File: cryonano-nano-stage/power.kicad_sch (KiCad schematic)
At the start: 1 part, among them J1 Conn_01x03_Pin

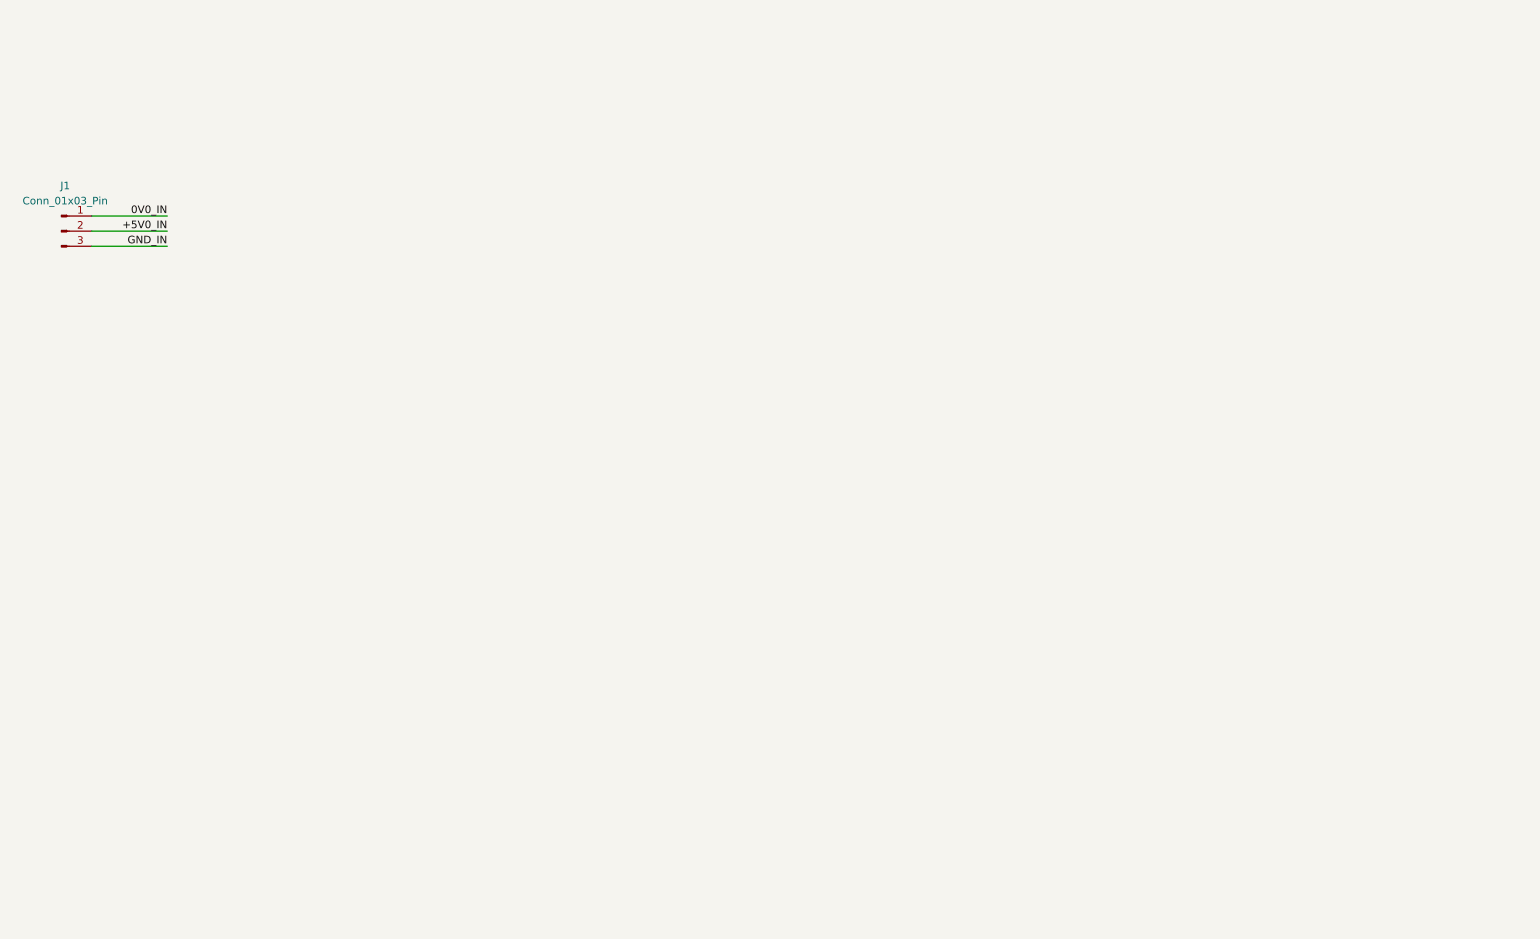
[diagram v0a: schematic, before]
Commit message: preliminary components added
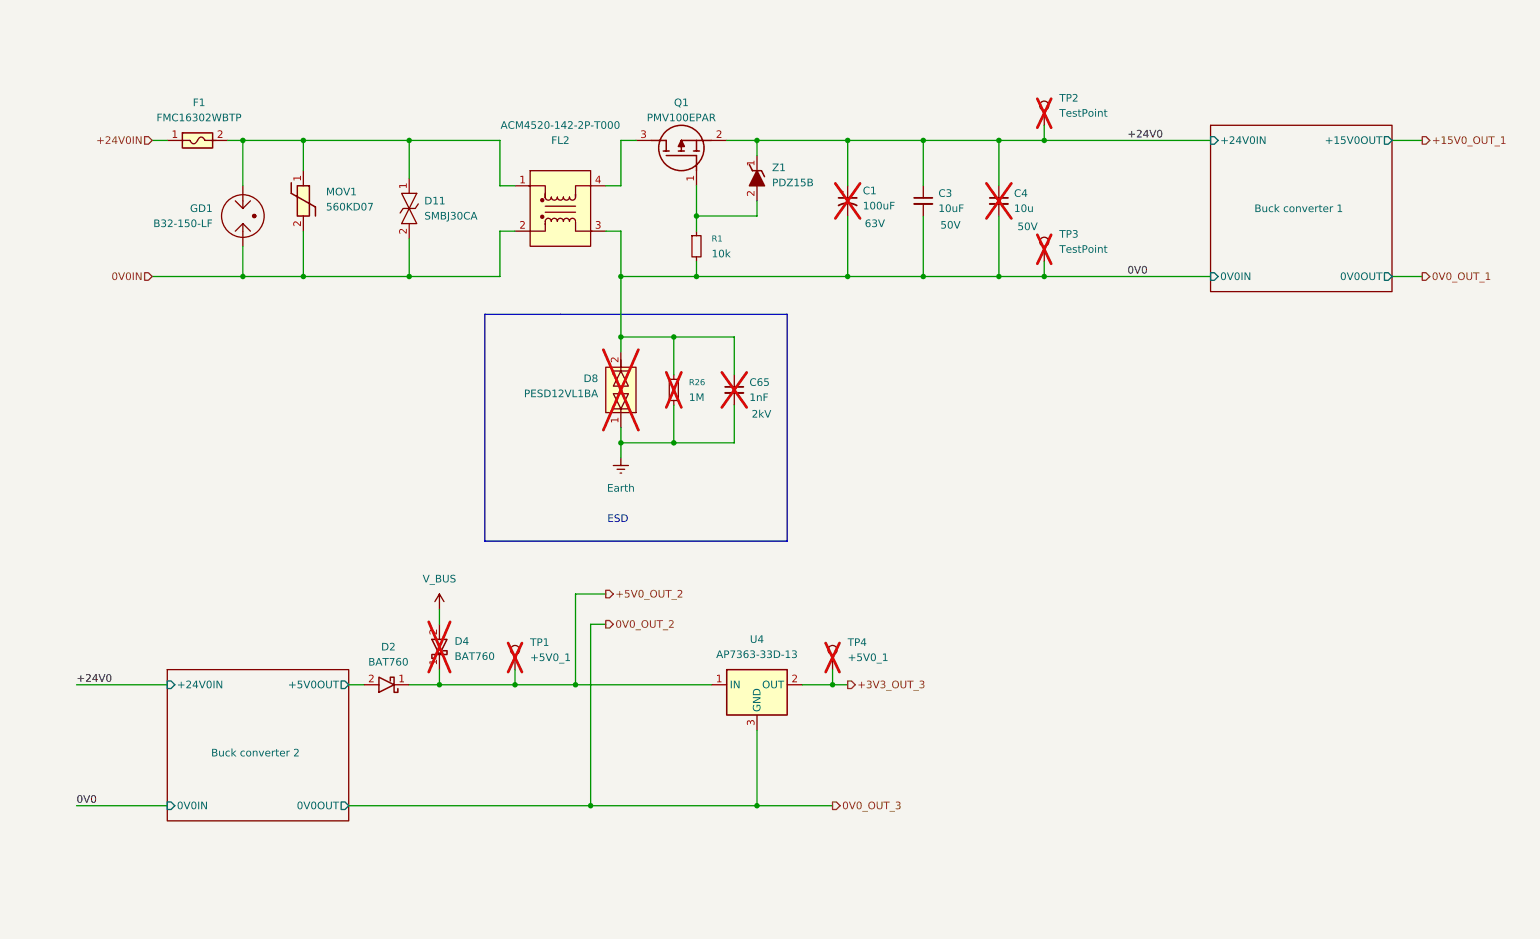
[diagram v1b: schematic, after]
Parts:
- removed J1: Conn_01x03_Pin, symbol Connector:Conn_01x03_Pin
- added C1: 100uF, Capacitor_THT:CP_Radial_D8.0mm_P3.50mm, symbol Device:C_Polarized_Small_US
- added C3: 10uF, Capacitor_SMD:C_1210_3225Metric, symbol Device:C_Small
- added C4: 10u, Capacitor_SMD:C_1206_3216Metric, symbol Device:C_Small
- added C65: 1nF, Capacitor_THT:C_Disc_D9.0mm_W5.0mm_P10.00mm, symbol Device:C_Small
- added D11: SMBJ30CA, Diode_SMD:D_SMB, symbol symbols:SMBJ30CA/TR13
- added D2, D4: BAT760, Diode_SMD:D_SOD-323, symbol symbols:BAT760
- added D8: PESD12VL1BA, Diode_SMD:D_SOD-323F, symbol symbols:PESD12VL1BA,115
- added F1: FMC16302WBTP, FUSC1608X55N, symbol symbols:FMC16302WBTP
- added FL2: ACM4520-142-2P-T000, footprints:ACM45204212PT000, symbol symbols:ACM4520-142-2P-T000
- added GD1: B32-150-LF, footprints:B32_GDT_YAGEO, symbol symbols:B32-150-LF
- added MOV1: 560KD07, Varistor:RV_Disc_D9mm_W4.8mm_P5mm, symbol symbols:560KD07
- added Q1: PMV100EPAR, footprints:SOT95P230X110-3N, symbol symbols:PMV100EPAR
- added R1: 10k, Resistor_SMD:R_0603_1608Metric, symbol Device:R_Small
- added R26: 1M, Resistor_THT:R_Axial_DIN0207_L6.3mm_D2.5mm_P10.16mm_Horizontal, symbol Device:R_Small
- added TP1, TP4: +5V0_1, footprints:TestPoint_THTPad_D1.3mm_Drill0.8mm, symbol Connector:TestPoint
- added TP2, TP3: TestPoint, footprints:TestPoint_THTPad_D1.3mm_Drill0.8mm, symbol Connector:TestPoint
- added U4: AP7363-33D-13, footprints:TO252__DPAK__1, symbol symbols:AP7363-33D-13
- added Z1: PDZ15B, footprints:SOD2512X110N, symbol base_6in_24out_components:PDZ15B,115
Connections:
- new net: D11.1, F1.2, FL2.1, GD1.1, MOV1.1
- new net: FL2.4, Q1.3 (D)
- new net: Q1.1 (G), R1.1, Z1.2 (A)
- new net +24V0: C1.1, C3.1, C4.1, Q1.2 (S), TP2.1, Z1.1 (K)
- new net +24V0IN: F1.1
- new net +3V3_OUT_3: TP4.1, U4.2 (OUT)
- new net +5V0_OUT_2: D2.1 (K), D4.1 (K), TP1.1, U4.1 (IN)
- new net 0V0: C1.2, C3.2, C4.2, C65.1, D8.2, FL2.3, R1.2, R26.1, TP3.1
- new net 0V0IN: D11.2, FL2.2, GD1.2, MOV1.2
- new net 0V0_OUT_2: U4.3 (GND)
- new net Buck converter 2/+5V0OUT: D2.2 (A)
- new net Earth: C65.2, D8.1, R26.2
- new net V_BUS: D4.2 (A)
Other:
- added sheet Buck converter 1 (buck-converter-1.kicad_sch)
- added sheet Buck converter 2 (buck-converter-2.kicad_sch)
- note added: "ESD"

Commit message: sch updated
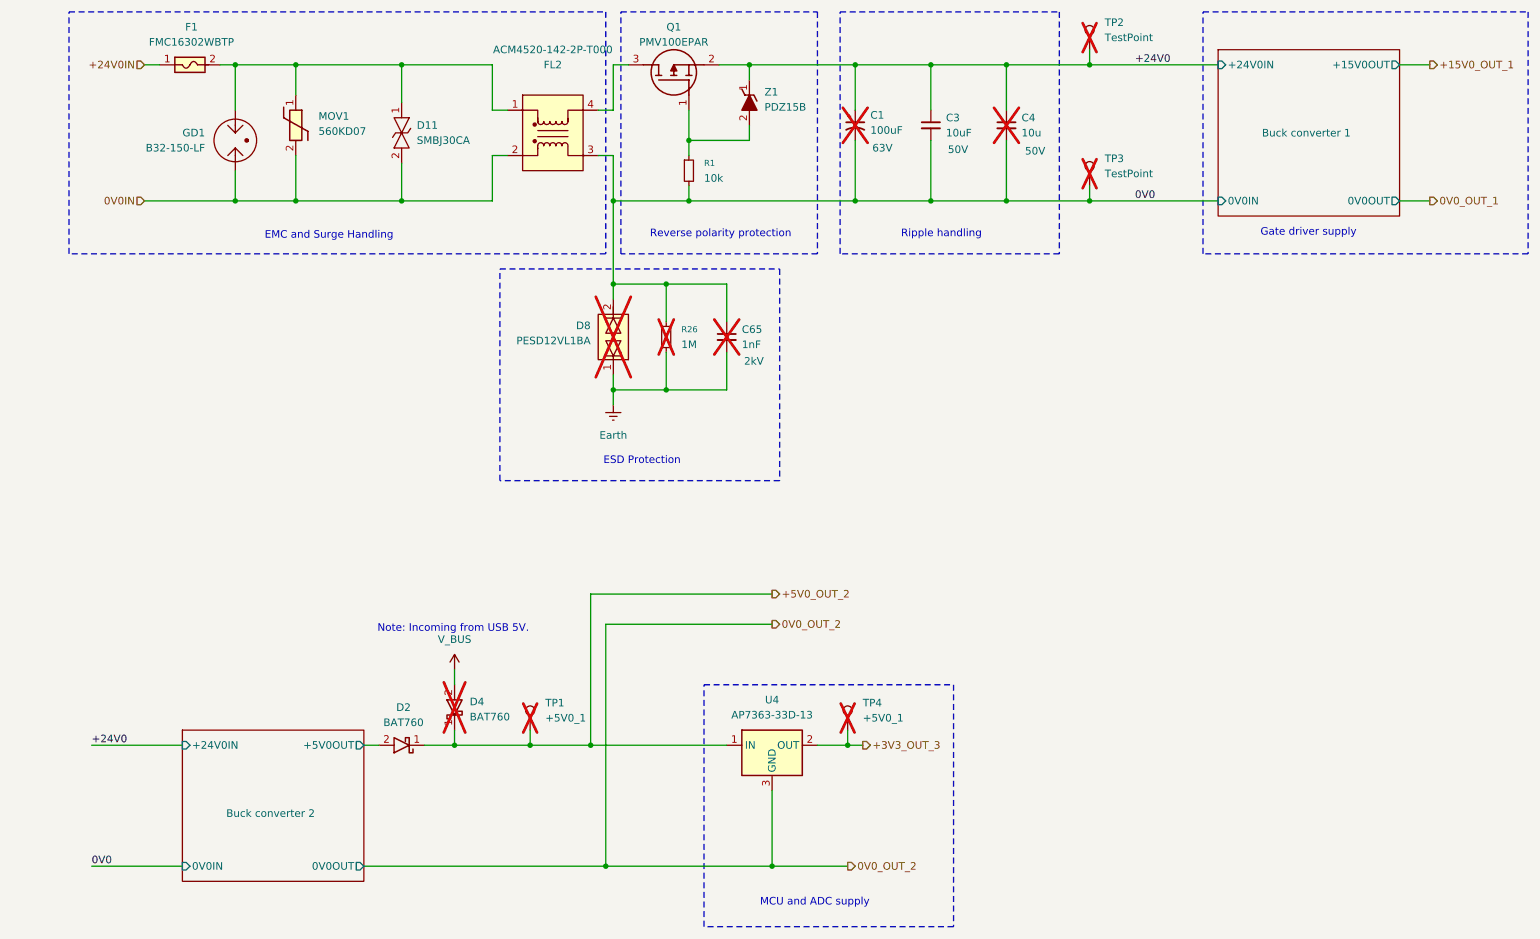
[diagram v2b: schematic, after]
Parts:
- FL2: Unit Price 10 109 -> 71
- U4: Order No. (none) -> AP7363-33D-13; Unit Price 10 (none) -> 27
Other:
- note added: "EMC and Surge Handling"
- note added: "ESD Protection"
- note added: "Gate driver supply"
- note added: "MCU and ADC supply"
- note added: "Note: Incoming from USB 5V."
- note added: "Reverse polarity protection"
- note added: "Ripple handling"
- note removed: "ESD"
- moved on the sheet: C1, C3, C4, C65, D11, D2, D4, D8, F1, FL2, GD1, MOV1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
